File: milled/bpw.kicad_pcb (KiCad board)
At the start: 2 copper layers, 13.5 x 10.2 mm, 6 parts, among them U1 ZXSC380

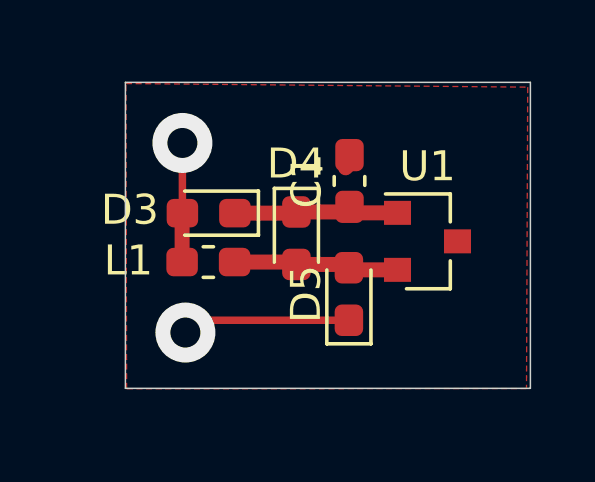
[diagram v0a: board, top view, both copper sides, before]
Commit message: Joule Thief
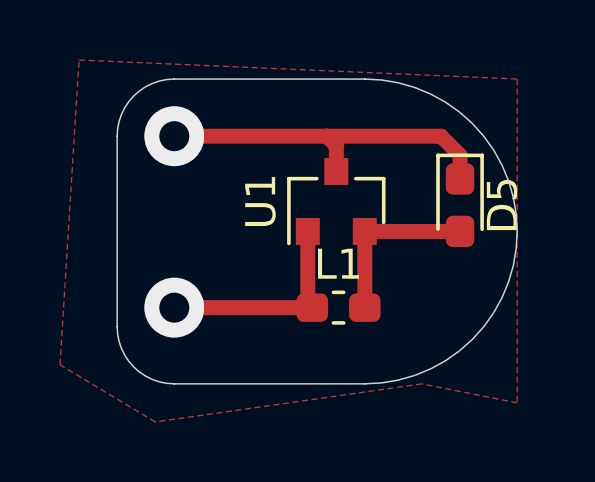
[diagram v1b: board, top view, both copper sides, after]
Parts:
- removed C1: 1uF, Capacitor_SMD:C_0603_1608Metric_Pad1.08x0.95mm_HandSolder
- removed D3, D4: D_Schottky, Diode_SMD:D_0603_1608Metric_Pad1.05x0.95mm_HandSolder
- moved D5 4.74 mm to (120.0, 74.1), turned to 270 degrees
- moved L1 4.60 mm to (116.0, 77.5)
- moved U1 3.32 mm to (115.9, 73.9), turned to 90 degrees
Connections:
- net GND renamed Net-(D2-Pad1)
- U1 pad 1: Net-(C1-Pad1) -> Net-(D1-Pad2)
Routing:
- net Net-(D2-Pad1): track 5.85 -> 11.9 mm
- net Net-(C1-Pad1): track 5.77 -> 0.00 mm
- net Net-(D1-Pad2): track 3.97 -> 7.20 mm
- added copper zone on F.Cu, net (none)
- removed copper zone on F.Cu, net Net-(D2-Pad1)
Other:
- board size 13.5 x 10.2 mm -> 13.3 x 10.2 mm
